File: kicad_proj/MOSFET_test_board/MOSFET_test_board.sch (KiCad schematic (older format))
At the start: 48 parts, among them J1 _GENERIC_CONNECTOR_01x02, J2 _GENERIC_CONNECTOR_01x03, J3 Tag_Connect_Programmer_6-Pin, J4 _GENERIC_CONNECTOR_01x02, Q1 AOD424, U1 STM32F401CCU6TR, U2 MCP1826ST-3302E_DB, U3 MIC4416YM4-TR, Y1 RH100-12.000-10-2020-EXT-TR

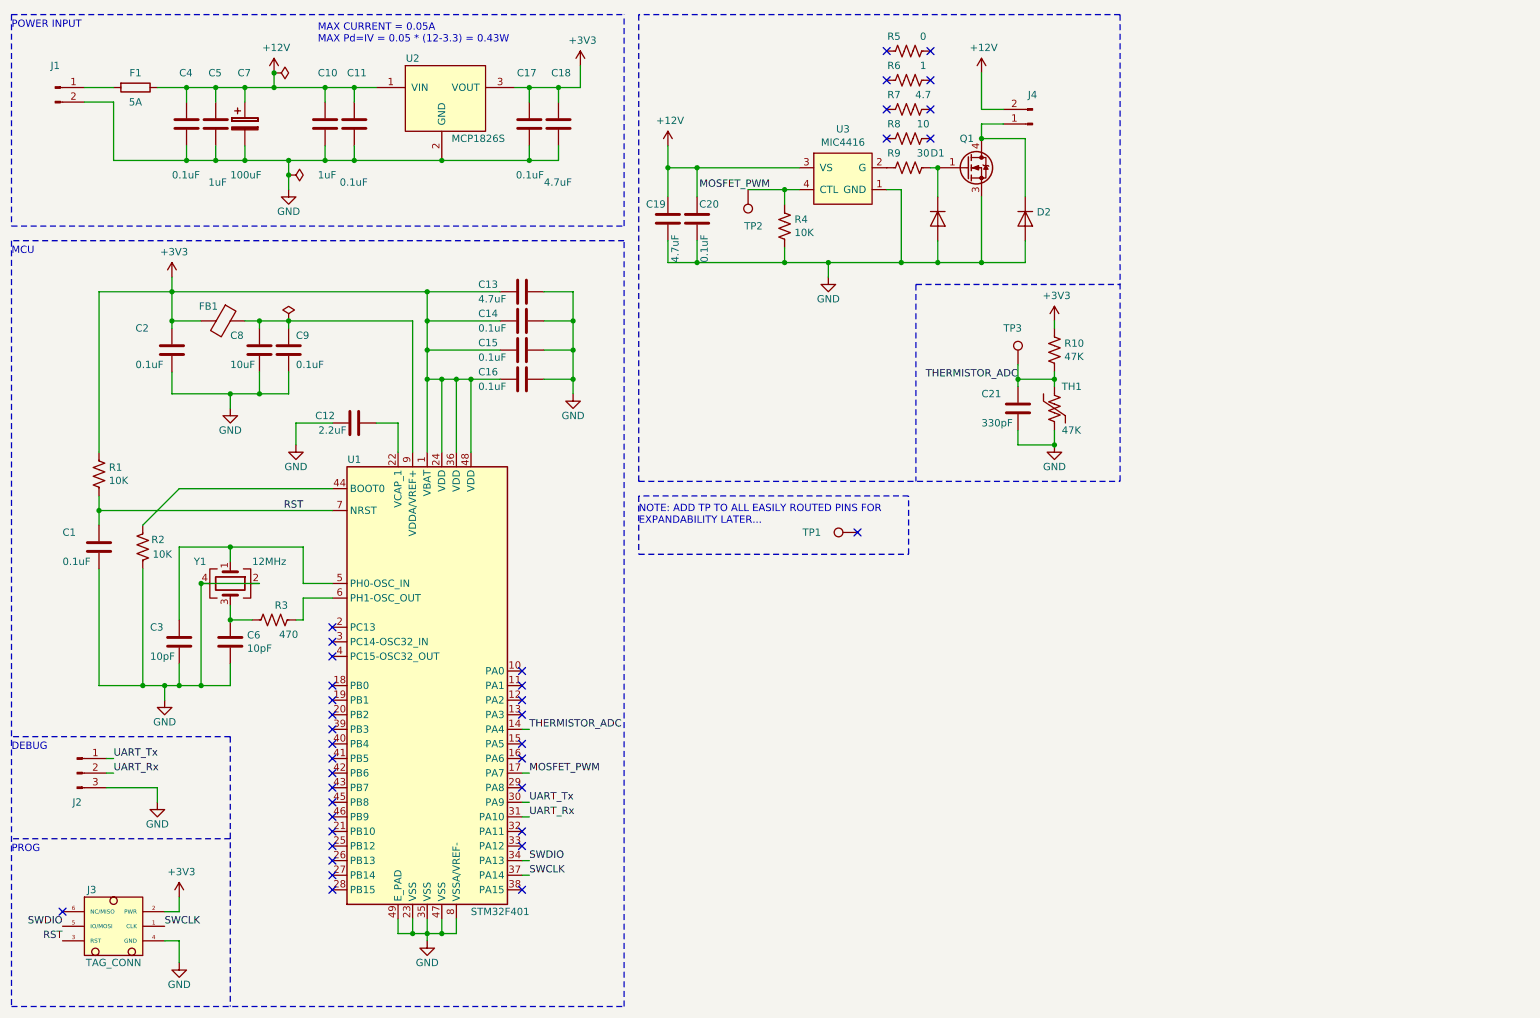
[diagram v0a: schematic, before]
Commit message: Fab outputs
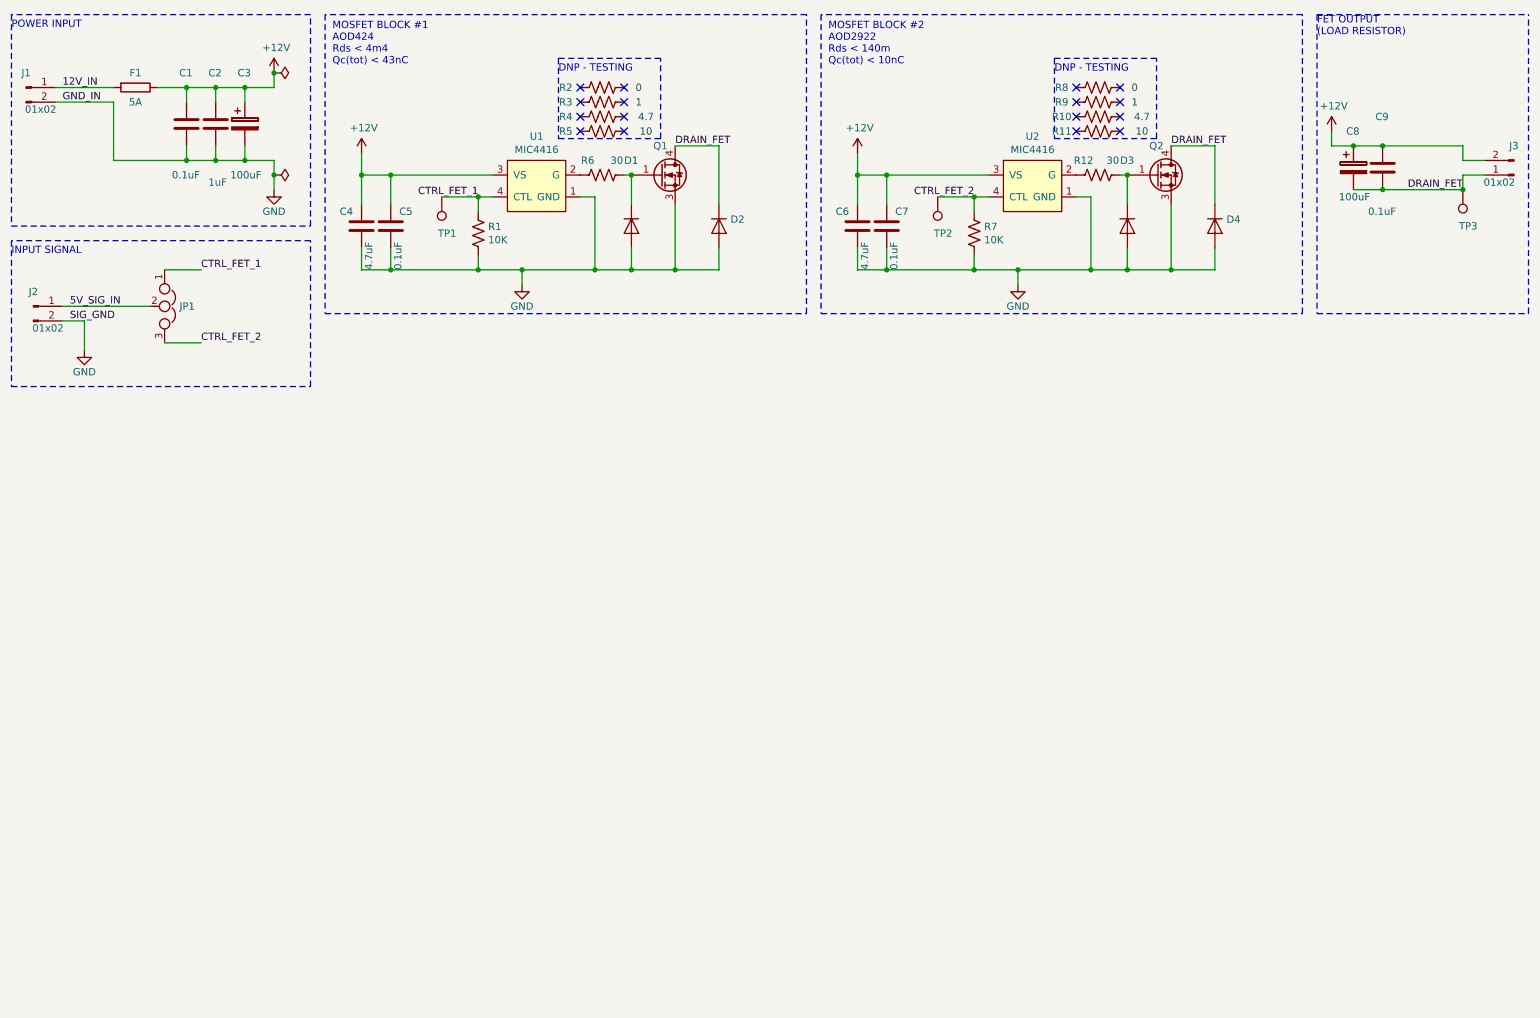
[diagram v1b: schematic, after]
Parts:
- removed C1, C11, C14, C15, C16, C17, C2: CL10B104KC8NNNC, footprints:CAPACITOR_0603N, symbol capacitors:CL10B104KC8NNNC
- removed C10: CL31B105KCHNNNE, footprints:CAPACITOR_1206N, symbol capacitors:CL31B105KCHNNNE
- removed C12: EMK107BB7225MA-T, symbol capacitors:EMK107BB7225MA-T
- removed C13, C18: CL10A475KA8NQNC, footprints:CAPACITOR_0603N, symbol capacitors:CL10A475KA8NQNC
- removed C21: CL10B331KB8NNNC, footprints:CAPACITOR_0603N, symbol capacitors:CL10B331KB8NNNC
- removed C3, C6: CC0402FRNPO9BN100, footprints:CAPACITOR_0402N, symbol capacitors:CC0402FRNPO9BN100
- removed C8: CL31A106KPHNNNE, footprints:CAPACITOR_1206N, symbol capacitors:CL31A106KPHNNNE
- removed FB1: 742792040, footprints:INDUCTOR_0805N, symbol inductors:742792040
- removed J1, J4: _GENERIC_CONNECTOR_01x02, symbol connectors:_GENERIC_CONNECTOR_01x02
- removed J2: _GENERIC_CONNECTOR_01x03, symbol connectors:_GENERIC_CONNECTOR_01x03
- removed J3: Tag_Connect_Programmer_6-Pin, symbol connectors:Tag_Connect_Programmer_6-Pin
- removed R1, R2: RC0603JR-0710KL, footprints:RESISTOR_0603N, symbol resistors:RC0603JR-0710KL
- removed R10: RC0603JR-0747KL, footprints:RESISTOR_0603N, symbol resistors:RC0603JR-0747KL
- removed R3: RC0603JR-07470RL, footprints:RESISTOR_0603N, symbol resistors:RC0603JR-07470RL
- removed TH1: NXFT15WB473FA2B150, symbol thermistors:NXFT15WB473FA2B150
- removed TP1: TestPoint, symbol Connector:TestPoint
- removed U1: STM32F401CCU6TR, footprints:QFN49P50_700X700X60L40X25T560N, symbol ics:STM32F401CCU6TR
- removed U2: MCP1826ST-3302E_DB, footprints:SOT223-4P230_700X180L87X72N, symbol ics:MCP1826ST-3302E_DB
- removed Y1: RH100-12.000-10-2020-EXT-TR, footprints:RH100-12.000-10-2020-EXT-TR, symbol misc:RH100-12.000-10-2020-EXT-TR
- added C6: CL10A475KA8NQNC, footprints:CAPACITOR_0603N, symbol capacitors:CL10A475KA8NQNC
- added C7: CL10B104KC8NNNC, footprints:CAPACITOR_0603N, symbol capacitors:CL10B104KC8NNNC
- added C8: EMVE160ADA101MF55G, footprints:CAPAE660X550D720L265X65N, symbol capacitors:EMVE160ADA101MF55G
- added D3, D4: SMAJ12A, footprints:DIODE_SMAN, symbol diodes:SMAJ12A
- added J1, J2, J3: 009296002202906, footprints:009296002202906, symbol connectors:009296002202906
- added JP1: Jumper_NC_Dual, Connector_PinHeader_2.54mm:PinHeader_1x03_P2.54mm_Vertical, symbol Device:Jumper_NC_Dual
- added Q2: AOD2922, footprints:DPAK3P457_994X240L165X76T538X492N, symbol mosfets:AOD2922
- added R10: SR0603FR-7T4R7L, symbol resistors:SR0603FR-7T4R7L
- added R11: SR0603FR-7T10RL, symbol resistors:SR0603FR-7T10RL
- added R12: RC0603JR-0730RL, footprints:RESISTOR_0603N, symbol resistors:RC0603JR-0730RL
- added R7: RC0603JR-0710KL, footprints:RESISTOR_0603N, symbol resistors:RC0603JR-0710KL
- added R8: RC0603JR-070RL, symbol resistors:RC0603JR-070RL
- added R9: SR0603FR-7T1RL, symbol resistors:SR0603FR-7T1RL
- added TP2: TestPoint, TestPoint:TestPoint_Pad_1.0x1.0mm, symbol Connector:TestPoint
- added U2: MIC4416YM4-TR, footprints:SOT143-4P190_237X112L31X44N, symbol ics:MIC4416YM4-TR
- F1: footprint (none) -> footprints:FUSE_0603N
- R2: renamed from R5; footprint footprints:RESISTOR_0603N -> (none)
- R3: renamed from R6; footprint footprints:RESISTOR_0603N -> (none)
- R4: renamed from R7; footprint footprints:RESISTOR_0603N -> (none)
- R5: renamed from R8; footprint footprints:RESISTOR_0603N -> (none)
- TP1: renamed from TP2; footprint (none) -> TestPoint:TestPoint_Pad_1.0x1.0mm
- TP3: footprint (none) -> TestPoint:TestPoint_Pad_1.0x1.0mm
- renumbered C4 to C1, C5 to C2, C7 to C3, C19 to C4, C20 to C5, R4 to R1, R9 to R6, U3 to U1
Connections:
- net THERMISTOR_ADC is gone; now on net DRAIN_FET: TP3.1
- net +12V: now also C9.1, C6.1, C7.1, C8.1, J3.2 (Pin_2), U2.3 (VS)
- net GND: now also C6.2, C7.2, D3.A, D4.A, J1.2 (Pin_2), J2.2 (Pin_2), Q2.3 (S), R7.2, U2.1 (GND); no longer C9.1
- net 12V_IN: now reaches F1.2
- net 12V_IN: now also J1.1 (Pin_1)
- net DRAIN_FET: now reaches C9.2
- net DRAIN_FET: now also D2.C (K), Q1.4 (D), C8.2, D4.C (K), J3.1 (Pin_1), Q2.4 (D)
- net MOSFET_PWM renamed CTRL_FET_1
- net CTRL_FET_1: now also JP1.1
- new net: D3.C (K), Q2.1 (G), R12.1
- new net: R12.2, U2.2 (G)
- new net 5V_SIG_IN: J2.1 (Pin_1), JP1.2
- new net CTRL_FET_2: JP1.3, R7.1, TP2.1, U2.4 (CTL)
- no-connect marks 38 -> 16
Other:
- note added: "DNP - TESTING \n"
- note added: "FET OUTPUT\n(LOAD RESISTOR)"
- note added: "INPUT SIGNAL"
- note added: "MOSFET BLOCK #1\nAOD424\nRds < 4m4\nQc(tot) < 43nC\n"
- note added: "MOSFET BLOCK #2\nAOD2922\nRds < 140m\nQc(tot) < 10nC\n"
- note removed: "DEBUG"
- note removed: "MAX CURRENT = 0.05A\nMAX Pd=IV = 0.05 * (12-3.3) = 0.43W"
- note removed: "MCU"
- note removed: "NOTE: ADD TP TO ALL EASILY ROUTED PINS FOR\nEXPANDABILITY LATER..."
- note removed: "PROG"
- moved on the sheet: C4, C5, D1, D2, Q1, R1, R2, R3, R4, R5, R6, TP1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
